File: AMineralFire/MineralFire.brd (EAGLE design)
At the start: 110.5 x 100 mm, 76 parts, among them IC2 OP-AMP, IC3 7432D, Q10 20MHz, Q2 20MHz, Q3 200mA/40V, Q4 200mA/40V, Q5 200mA/40V, Q6 200mA/40V, Q7 200mA/40V, Q8 200mA/40V, Q9 200mA/40V, T1 600mA/40V, T2 600mA/40V, T3 600mA/40V, T4 600mA/40V, T5 600mA/40V, U3 +12v, U4 ATMEGA328P_TQFP, U5 ATMEGA328P_TQFP

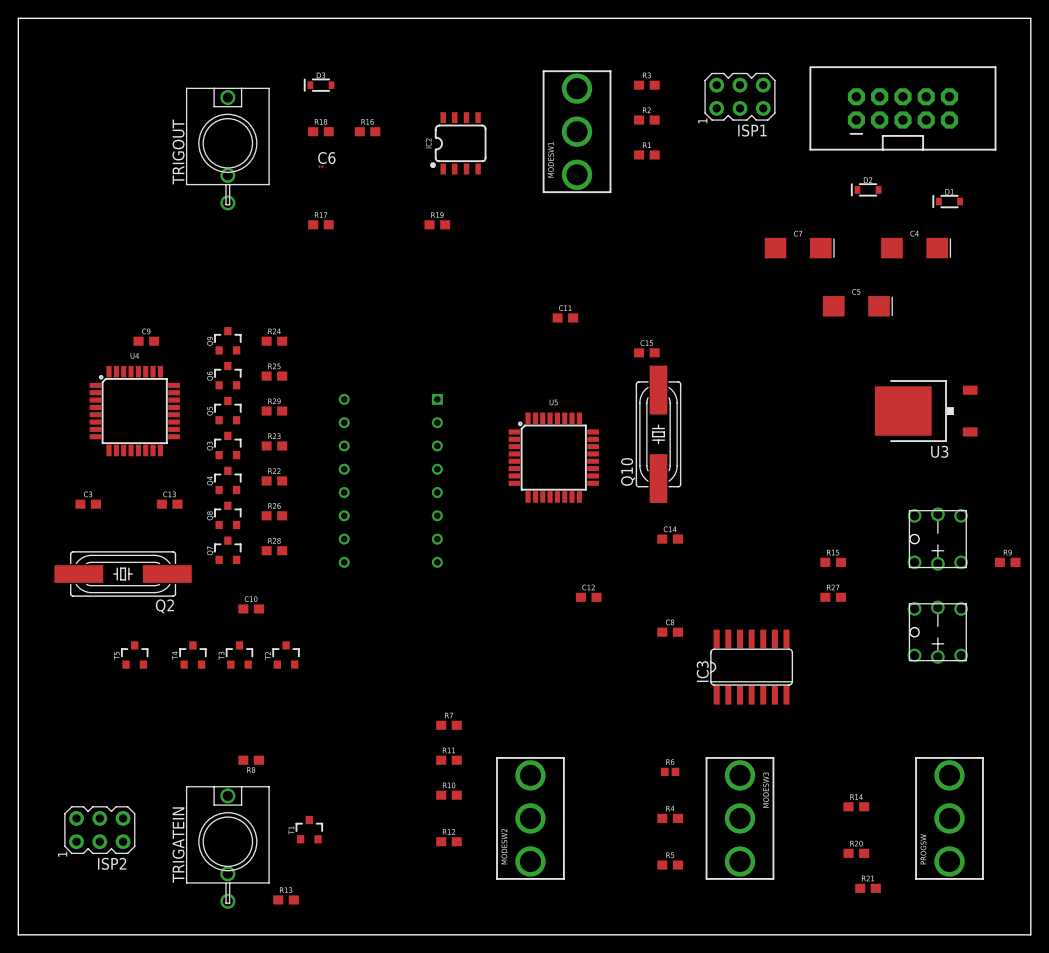
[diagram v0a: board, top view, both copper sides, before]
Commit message: first SMD
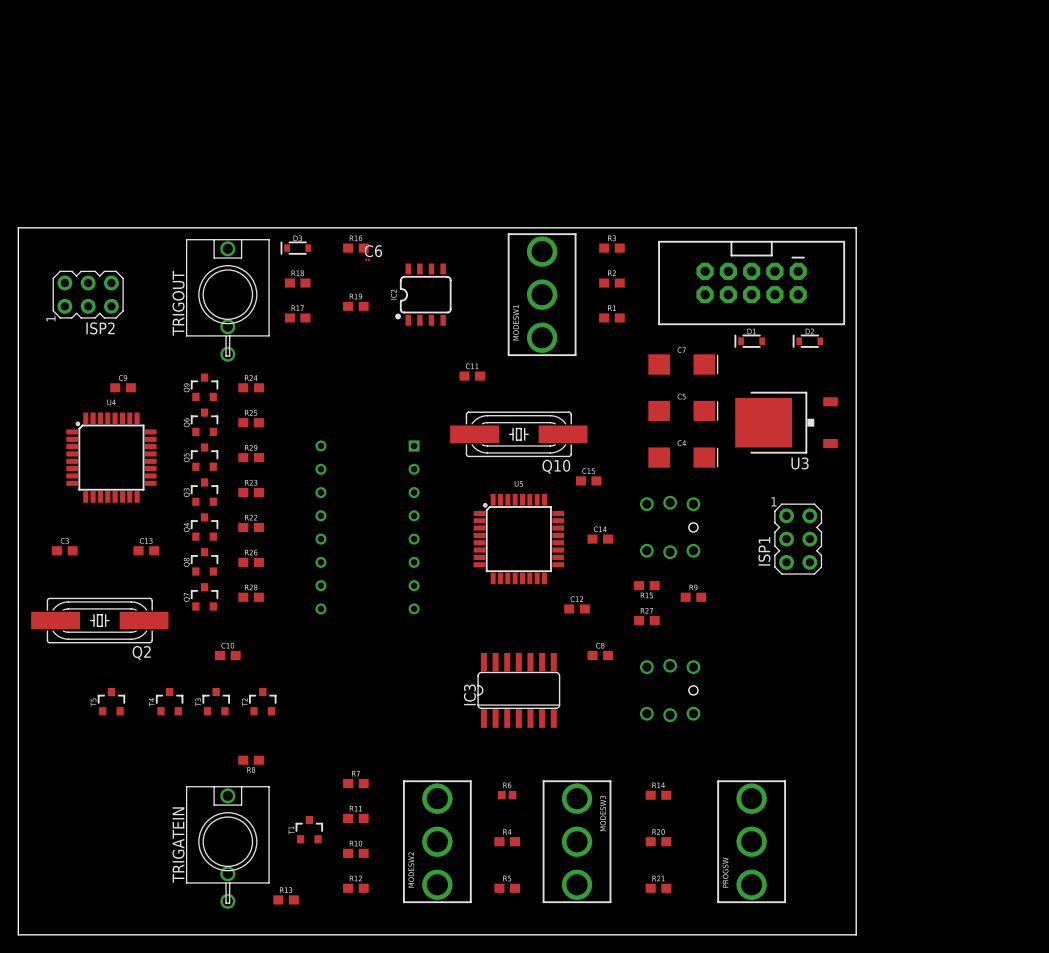
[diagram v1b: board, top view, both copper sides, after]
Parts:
- moved ISP2 58.4 mm to (7.62, 69.8)
- moved ISP1 48.7 mm to (85.1, 43.2), turned to 0 degrees
- moved R9 34.5 mm to (73.7, 36.8)
- moved C4 34.2 mm to (72.4, 52.1)
- moved BUT1 29.9 mm to (71.1, 26.7), flipped to the bottom
- moved BUT 29.2 mm to (71.1, 44.5), flipped to the bottom
- moved D1 26.4 mm to (80.0, 64.8)
- moved IC3 25.5 mm to (54.6, 26.7)
- moved POWER 25.2 mm to (80.0, 71.1), turned to 270 degrees
- moved R21 22.9 mm to (69.8, 5.08)
- moved C5 22.2 mm to (72.4, 57.1)
- moved PROGSW 21.7 mm to (80.0, 10.2)
- moved R14 21.6 mm to (69.8, 15.2)
- moved R20 21.6 mm to (69.8, 10.2)
- moved R15 20.5 mm to (68.6, 38.1), turned to 180 degrees
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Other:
- board size 110.5 x 100 mm -> 91.4 x 77.1 mm
